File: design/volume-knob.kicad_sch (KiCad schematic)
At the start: 35 parts, among them IC1 SGM2212-3.3XKC3G_TR, J1 USB_C_Receptacle, SW1 RotaryEncoder_Switch, SW2 SW_Push, SW3 SW_Push, U1 ESP32-C6-WROOM-1

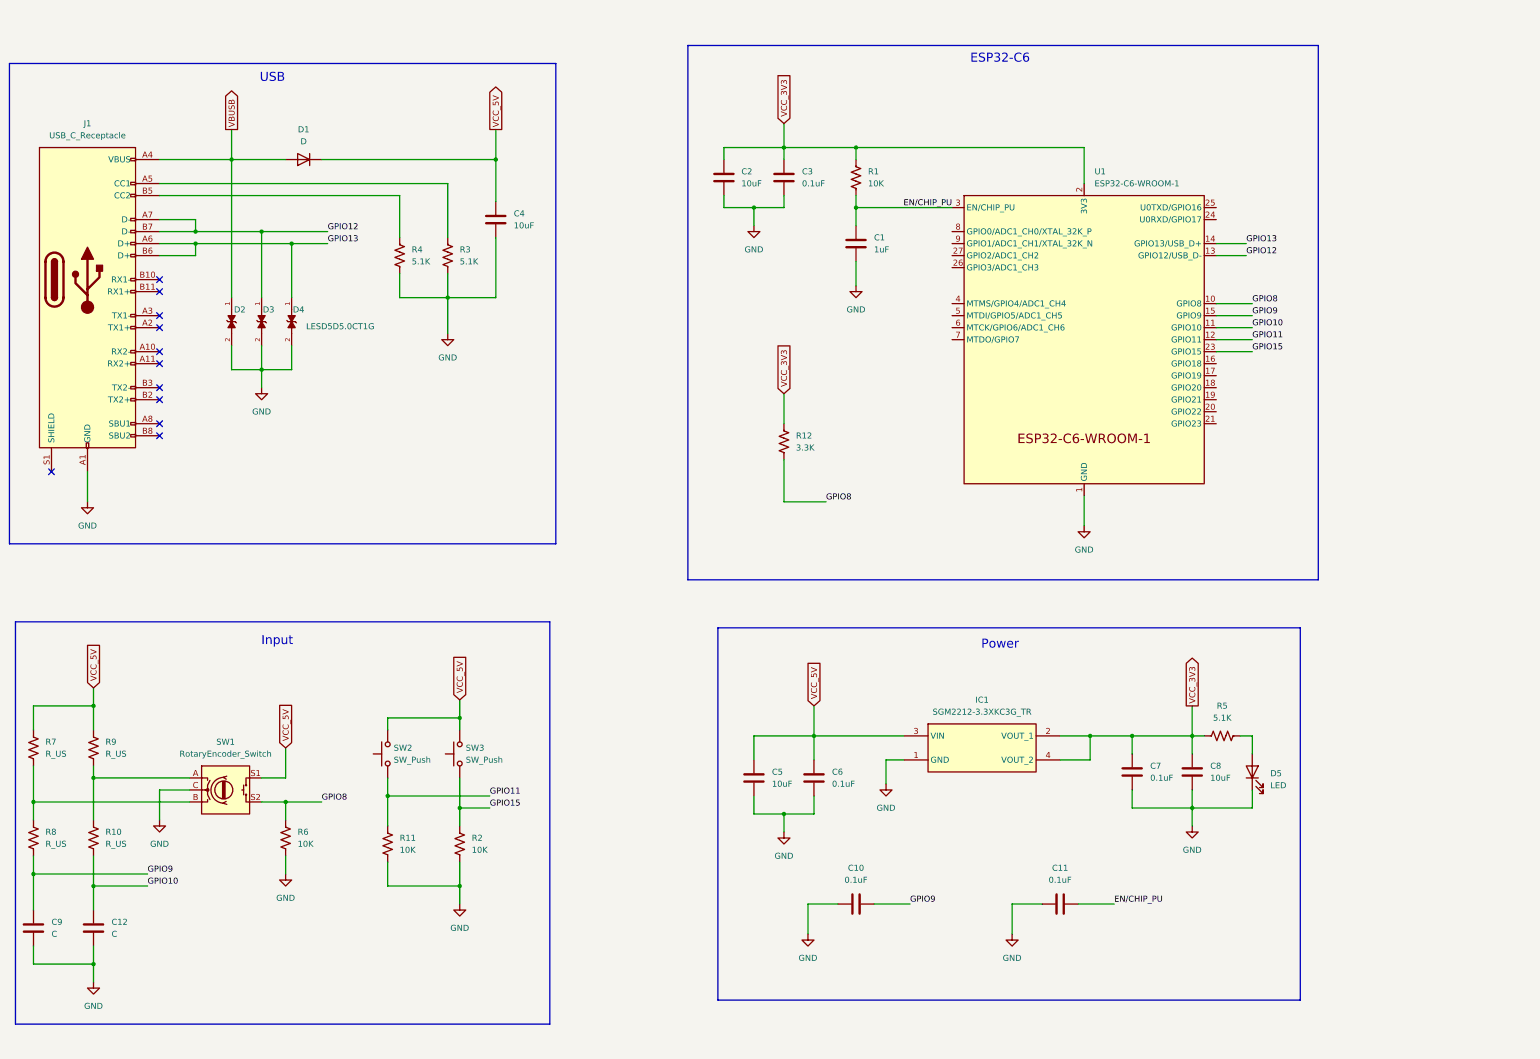
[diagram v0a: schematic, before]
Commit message: update kicad schematic and pcb
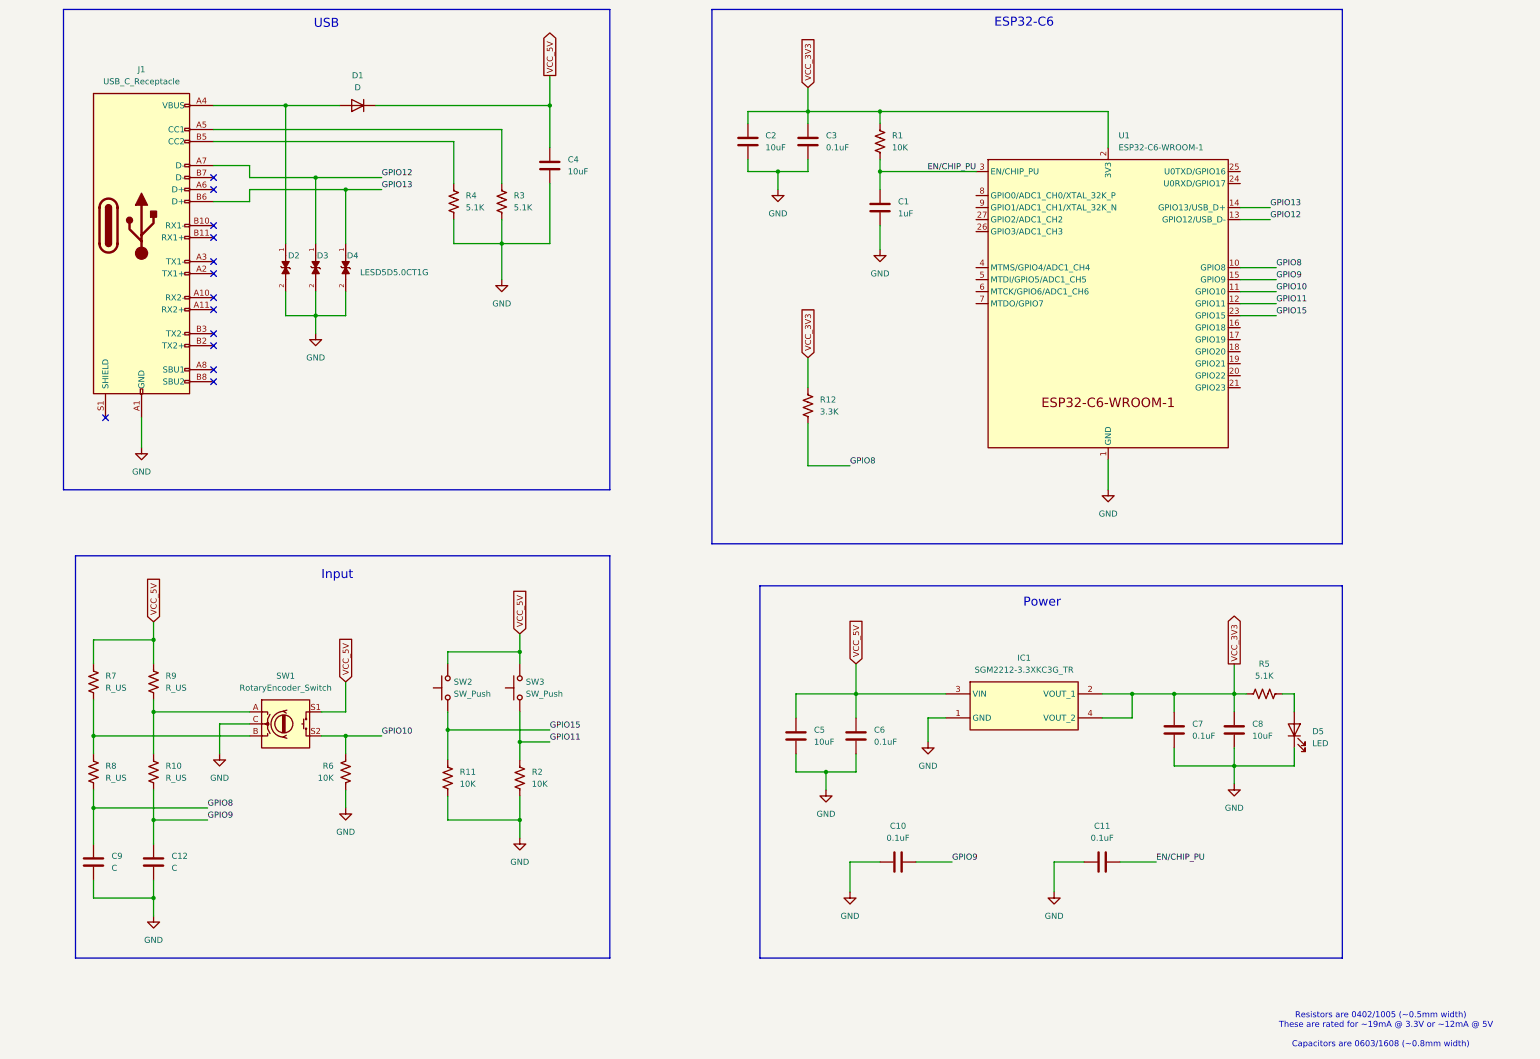
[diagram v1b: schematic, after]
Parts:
- C10, C11: footprint (none) -> Capacitor_SMD:C_0201_0603Metric
- J1: footprint Connector_USB:USB_C_Receptacle_Molex_105450-0101 -> Connector_USB:USB_C_Receptacle_GCT_USB4105-xx-A_16P_TopMnt_Horizontal
- R1, R10, R11, R2, R3, R4, R5, R6, R7, R8, R9: footprint Resistor_SMD:R_0201_0603Metric -> Resistor_SMD:R_01005_0402Metric
- R12: footprint (none) -> Resistor_SMD:R_01005_0402Metric
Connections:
- net GPIO10: now also R6.1, SW1.S2; no longer C12.1, R10.2
- net GPIO11: now also R2.2, SW3.1; no longer R11.2, SW2.1
- net GPIO12: no longer J1.B7 (D-)
- net GPIO13: no longer J1.A6 (D+)
- net GPIO15: now also R11.2, SW2.1; no longer R2.2, SW3.1
- net GPIO8: now also C9.1, R8.2; no longer R6.1, SW1.S2
- net GPIO9: now also C12.1, R10.2; no longer C9.1, R8.2
- net VBUSB: no longer names the net of D1.2 (A), D2.1, J1.A4 (VBUS), J1.A9 (VBUS), J1.B4 (VBUS), J1.B9 (VBUS)
- no-connect marks 11 -> 13
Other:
- note added: "Resistors are 0402/1005 (~0.5mm width) These are rated for ~19mA @ 3.3V or ~12mA @ 5V Capacitors are 0603/1608 (~0.8mm width)"
- moved on the sheet: C1, C10, C11, C12, C2, C3, C4, C5, C6, C7, C8, C9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
